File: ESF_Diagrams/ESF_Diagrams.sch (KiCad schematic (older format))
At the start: 91 parts, among them M1 Motor, M2 Motor, U2 AIR, U3 AIR

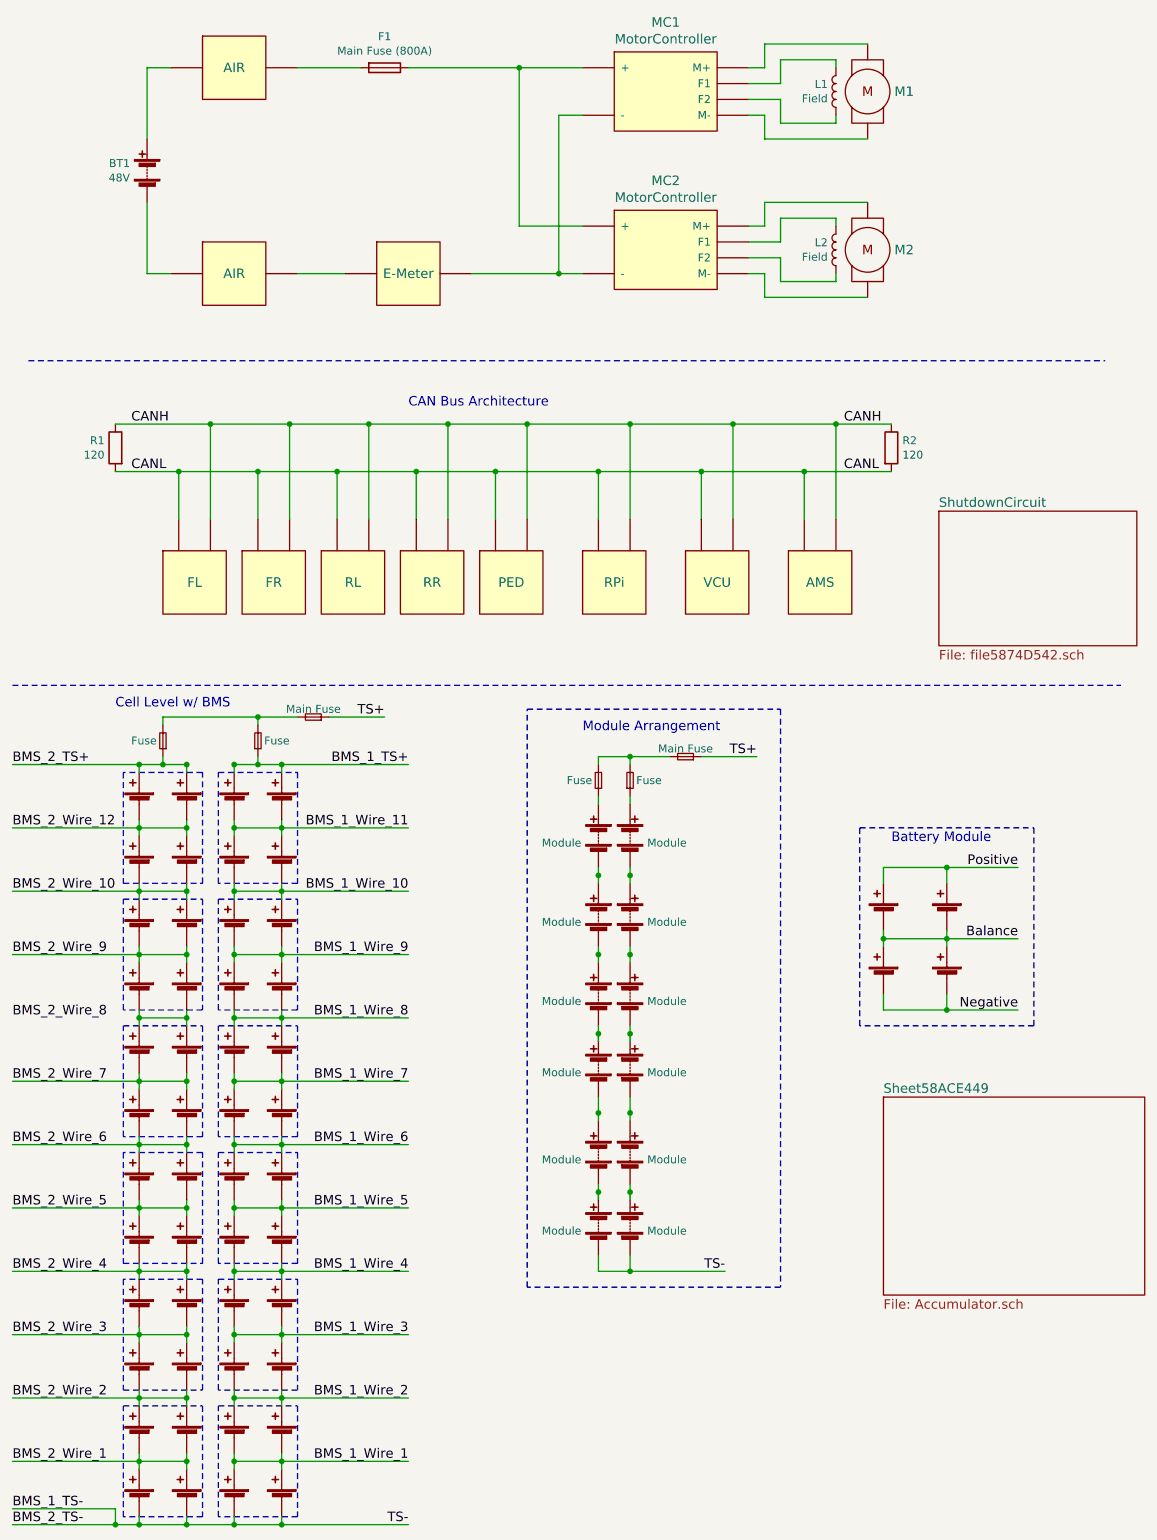
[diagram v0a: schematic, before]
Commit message: ESF Fixes
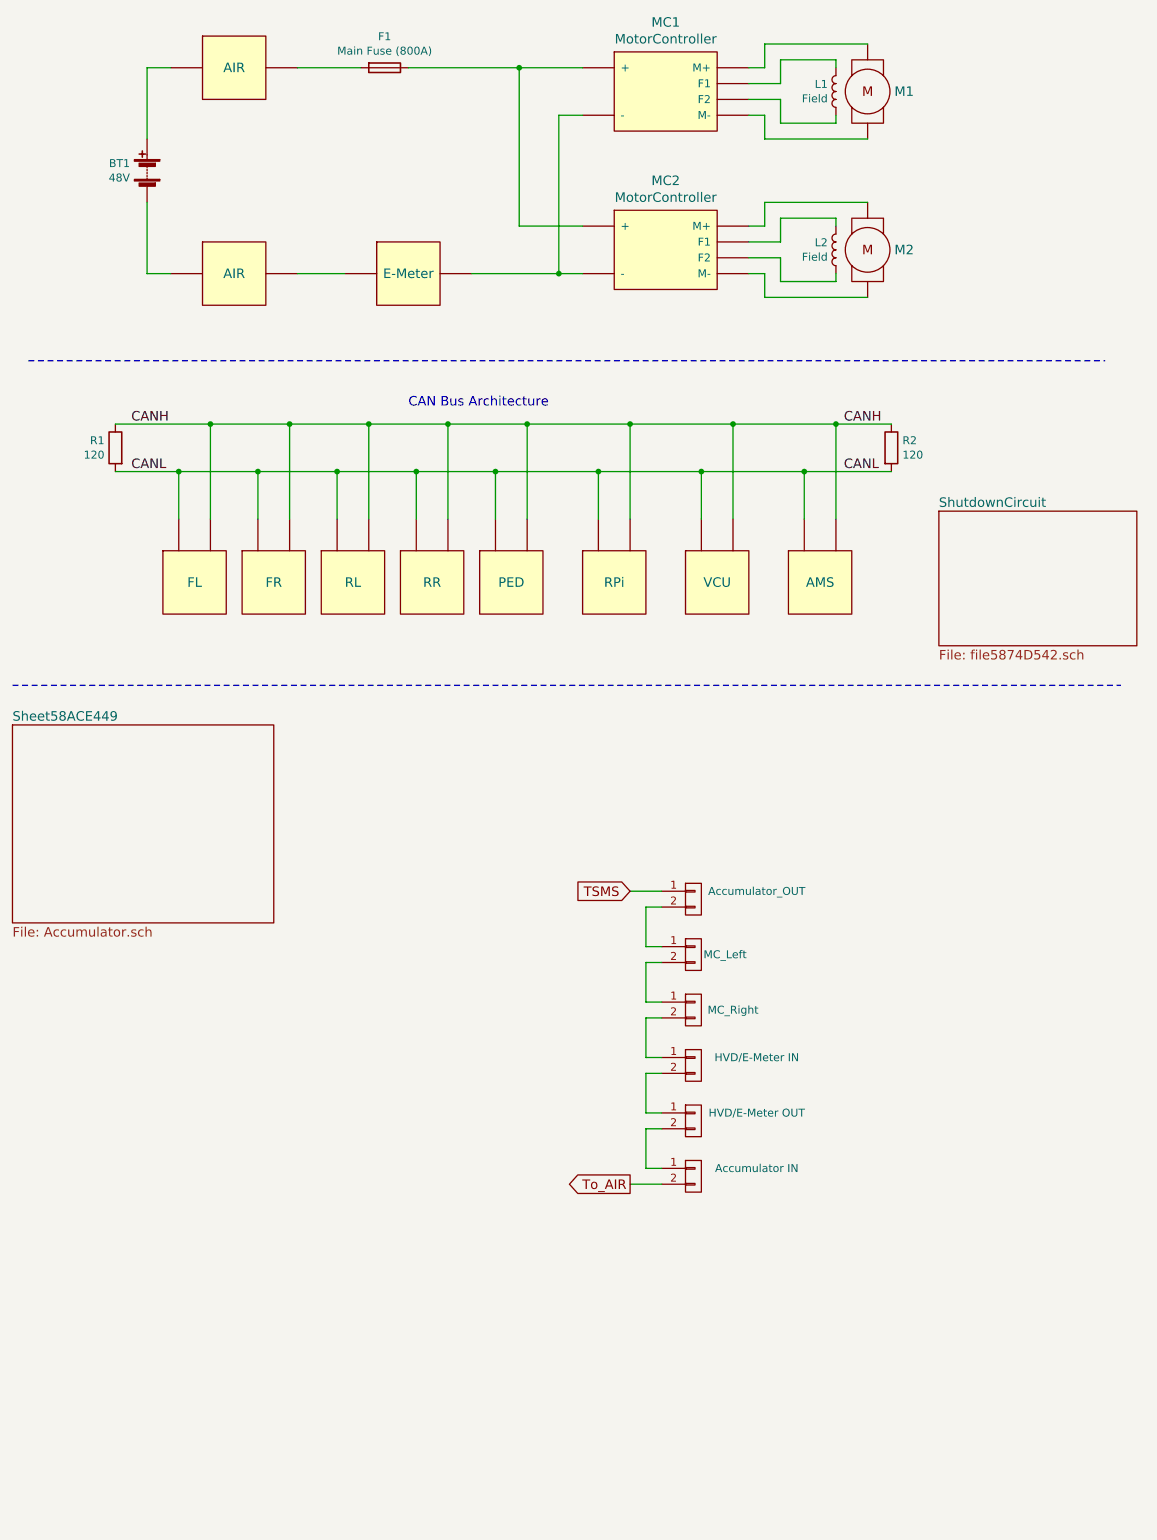
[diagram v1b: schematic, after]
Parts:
- removed BT? (x52): Battery_Cell, symbol Battery_Cell
- removed BT? (x12): Module, symbol Battery
- removed F? (x4): Fuse, symbol Fuse_Small
- removed F? (x2): Main Fuse, symbol Fuse_Small
- added J?: Accumulator_OUT, symbol CONN_01X02
- added J?: MC_Left, symbol CONN_01X02
- added J?: MC_Right, symbol CONN_01X02
- added J?: HVD/E-Meter IN, symbol CONN_01X02
- added J?: HVD/E-Meter OUT, symbol CONN_01X02
- added J?: Accumulator IN, symbol CONN_01X02
- gave numbers to parts that had none: 9
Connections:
- net at MC1.~ (M-): now also L1.2; no longer M1.~
- net at MC2.~ (M-): now also L2.2; no longer M2.~
- new net: F1.1, MC1.~ (M-), MC2.~ (M-)
- new net: MC1.~ (M-), MC2.~ (M-), U6.~
- new net: M1.~, MC1.~ (M-)
- new net: M2.~, MC2.~ (M-)
- new net: J?.1 (P1), J?.2 (P2) (x5)
- new net TSMS: J?.1 (P1)
- new net To_AIR: J?.2 (P2)
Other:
- note removed: "Battery Module"
- note removed: "Cell Level w/ BMS"
- note removed: "Module Arrangement"
